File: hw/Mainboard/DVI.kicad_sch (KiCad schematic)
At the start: 15 parts, among them J23 NOT_HDMI_A

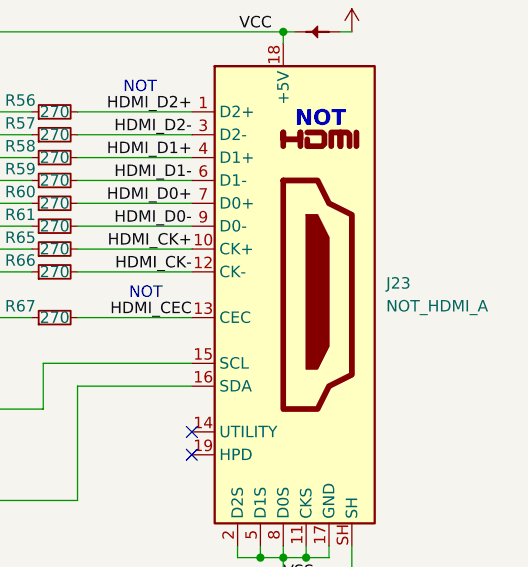
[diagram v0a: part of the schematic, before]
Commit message: hw: 25x2 header (wip)
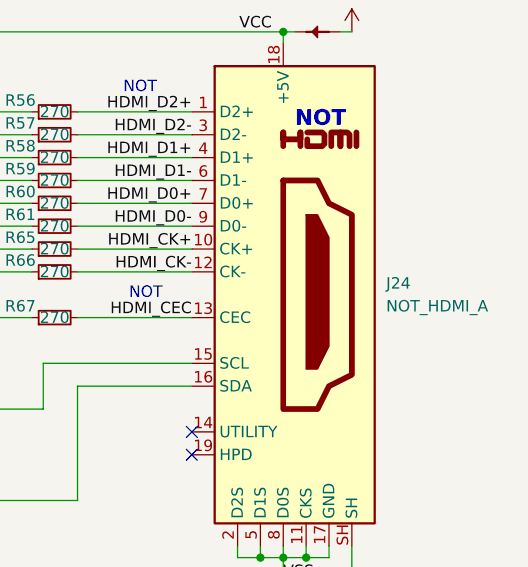
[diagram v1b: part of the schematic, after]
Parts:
- renumbered J23 to J24
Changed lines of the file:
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@@
   (symbol (lib_id "power:+5V") (at 198.12 59.69 0) (unit 1)
     (in_bom yes) (on_board yes) (fields_autoplaced)
-    (property "Reference" "#PWR0141" (id 0) (at 198.12 63.5 0)
+    (property "Reference" "#PWR0143" (id 0) (at 198.12 63.5 0)
       (effects (font (size 1.27 1.27)) hide)
     )
@@
   (symbol (lib_id "power:+3V3") (at 124.46 80.01 0) (mirror y) (unit 1)
     (in_bom yes) (on_board yes)
-    (property "Reference" "#PWR0142" (id 0) (at 124.46 83.82 0)
+    (property "Reference" "#PWR0144" (id 0) (at 124.46 83.82 0)
       (effects (font (size 1.27 1.27)) hide)
     )
@@
   (symbol (lib_id "Connector:HDMI_A") (at 190.5 88.9 0) (unit 1)
     (in_bom yes) (on_board yes)
-    (property "Reference" "J23" (id 0) (at 201.93 87.63 0)
+    (property "Reference" "J24" (id 0) (at 201.93 87.63 0)
       (effects (font (size 1.27 1.27)) (justify left))
     )
@@
   (symbol (lib_id "PET:PD_GND") (at 198.12 121.92 0) (unit 1)
     (in_bom yes) (on_board yes) (fields_autoplaced)
-    (property "Reference" "#PWR0143" (id 0) (at 198.12 128.27 0)
+    (property "Reference" "#PWR0145" (id 0) (at 198.12 128.27 0)
       (effects (font (size 1.27 1.27)) hide)
     )

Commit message: hw: 2x config switch (wip)
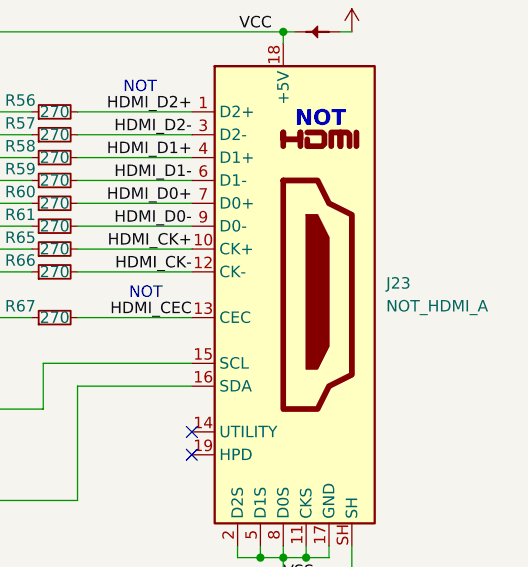
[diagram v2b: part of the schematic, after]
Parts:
- renumbered J24 to J23
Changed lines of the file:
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@@
   (symbol (lib_id "power:+5V") (at 198.12 59.69 0) (unit 1)
     (in_bom yes) (on_board yes) (fields_autoplaced)
-    (property "Reference" "#PWR0143" (id 0) (at 198.12 63.5 0)
+    (property "Reference" "#PWR0149" (id 0) (at 198.12 63.5 0)
       (effects (font (size 1.27 1.27)) hide)
     )
@@
   (symbol (lib_id "power:+3V3") (at 124.46 80.01 0) (mirror y) (unit 1)
     (in_bom yes) (on_board yes)
-    (property "Reference" "#PWR0144" (id 0) (at 124.46 83.82 0)
+    (property "Reference" "#PWR0150" (id 0) (at 124.46 83.82 0)
       (effects (font (size 1.27 1.27)) hide)
     )
@@
   (symbol (lib_id "Connector:HDMI_A") (at 190.5 88.9 0) (unit 1)
     (in_bom yes) (on_board yes)
-    (property "Reference" "J24" (id 0) (at 201.93 87.63 0)
+    (property "Reference" "J23" (id 0) (at 201.93 87.63 0)
       (effects (font (size 1.27 1.27)) (justify left))
     )
@@
   (symbol (lib_id "PET:PD_GND") (at 198.12 121.92 0) (unit 1)
     (in_bom yes) (on_board yes) (fields_autoplaced)
-    (property "Reference" "#PWR0145" (id 0) (at 198.12 128.27 0)
+    (property "Reference" "#PWR0151" (id 0) (at 198.12 128.27 0)
       (effects (font (size 1.27 1.27)) hide)
     )
